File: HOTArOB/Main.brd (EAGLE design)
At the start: 37 x 40.5 mm, 15 parts

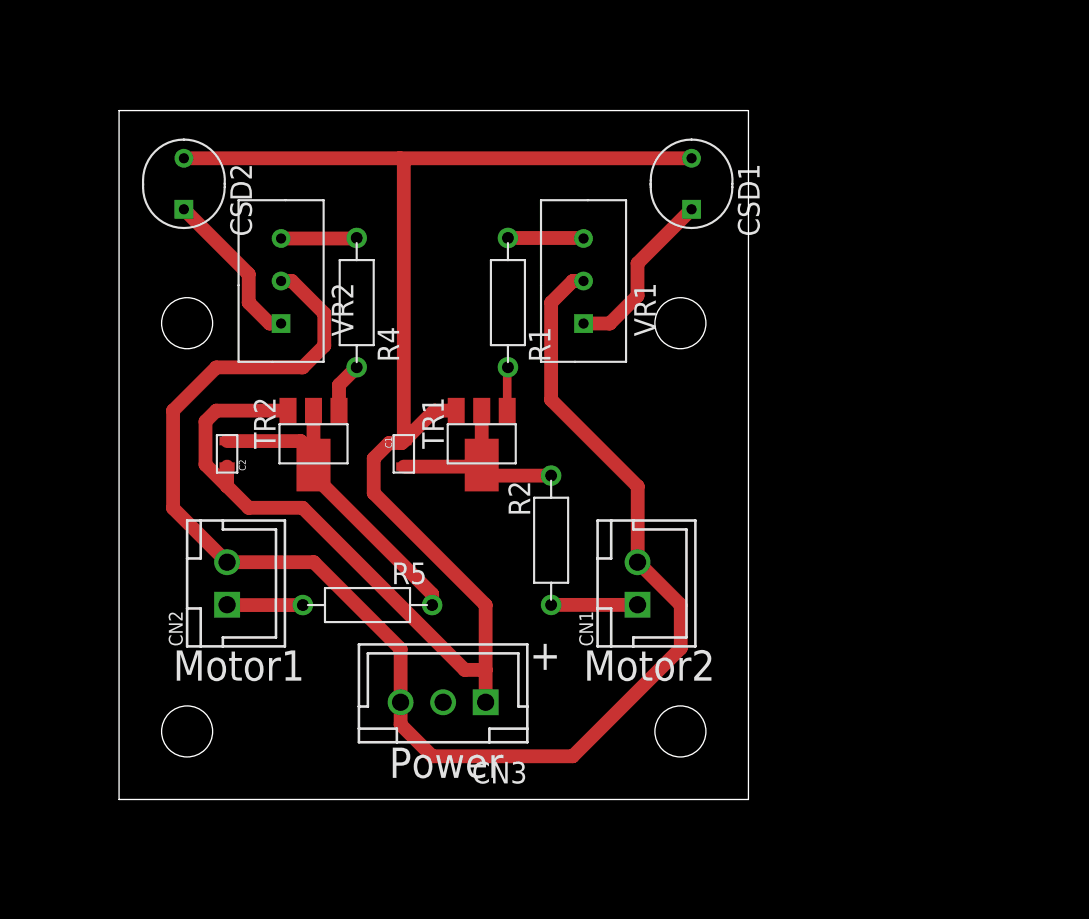
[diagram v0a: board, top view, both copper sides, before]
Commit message: working commit
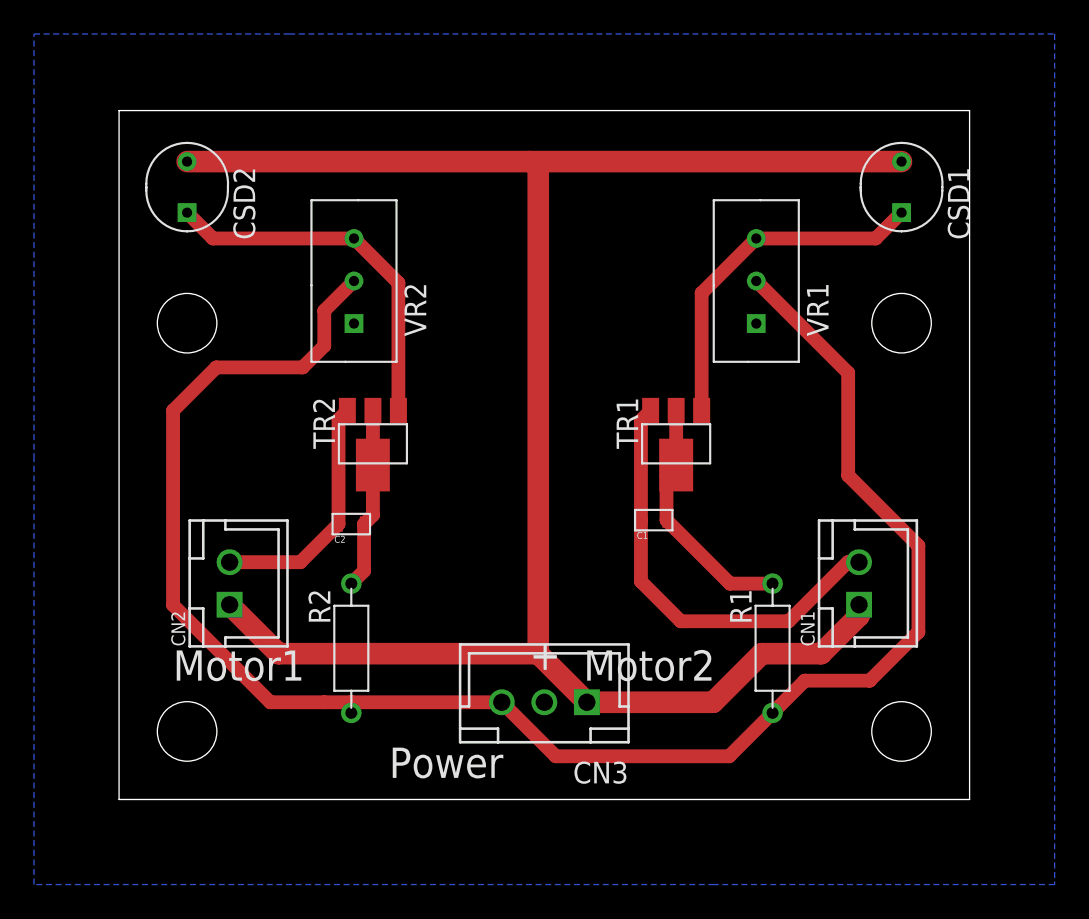
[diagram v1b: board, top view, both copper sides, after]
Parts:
- removed R4, R5: 1/4W_RESISTER, Tr_EXT:MF1/4
- moved R1 25.6 mm to (38.4, 8.89), turned to 270 degrees
- moved C1 15.2 mm to (31.4, 16.4), turned to 0 degrees
- moved R2 13.4 mm to (13.7, 8.89)
- moved CN1 13.0 mm to (43.5, 12.7)
- moved CSD1 12.3 mm to (46.0, 36.0)
- moved TR1 11.4 mm to (32.8, 22.9)
- moved VR1 10.2 mm to (37.5, 30.5)
- moved C2 8.39 mm to (13.7, 16.2), turned to 0 degrees
- moved CN3 5.95 mm to (25.0, 5.71)
- moved VR2 4.29 mm to (13.8, 30.5)
- moved TR2 3.49 mm to (14.9, 22.9)
- moved CSD2 0.27 mm to (4.00, 36.0)
- moved CN2 0.15 mm to (6.50, 12.7)
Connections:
- removed net N$10: R4.P$2, VR2.P$3
- removed net N$5: CN1.1, R2.P$2
- removed net N$6: CN2.1, R5.P$2
- removed net N$7: CSD2.P$1, VR2.P$1
- net GND: now also R1.P$2, R2.P$2; no longer CN1.2, CN2.2
- net N$1: now also C1.P$1, CN1.2, TR1.E; no longer R1.P$1, TR1.B
- net N$2: now also R1.P$1; no longer R2.P$1
- net N$3: now also C2.P$1, CN2.2, TR2.E; no longer CSD1.P$1, VR1.P$1
- net N$4: now also R2.P$1; no longer R5.P$1
- net N$8: now also CSD2.P$1, VR2.P$3; no longer R4.P$1
- net N$9: now also CSD1.P$1, TR1.B; no longer R1.P$2
- net VCC: now also CN1.1, CN2.1; no longer C1.P$1, C2.P$1, TR1.E, TR2.E
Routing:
- net N$1: track 2.57 -> 25.5 mm
- net N$8: track 2.98 -> 21.9 mm
- net N$9: track 4.46 -> 20.6 mm
- net GND: track 88.5 -> 102.2 mm
- net VCC: track 100.2 -> 113.4 mm
- net N$4: track 20.4 -> 10.7 mm
- net N$7: track 9.48 -> 0.00 mm
- net N$5: track 5.08 -> 0.00 mm
- net N$6: track 4.46 -> 0.00 mm
- net N$10: track 4.46 -> 0.00 mm
- net N$3: track 10.2 -> 14.2 mm
- net N$2: track 13.2 -> 14.5 mm
- added copper zone on layer 16, net GND
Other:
- board size 37 x 40.5 mm -> 50 x 40.5 mm
